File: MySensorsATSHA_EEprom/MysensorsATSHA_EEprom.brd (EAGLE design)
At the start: 22.1 x 12.1 mm, 3 parts, among them IC1 AT25DF512C-SSHN-B

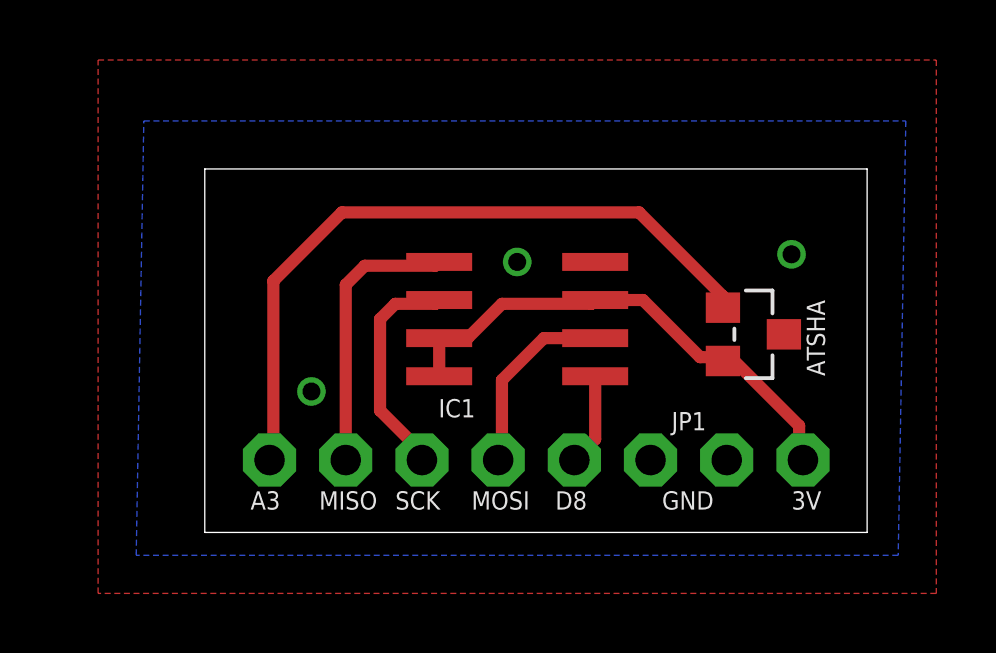
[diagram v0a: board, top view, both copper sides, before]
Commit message: routing minor changes
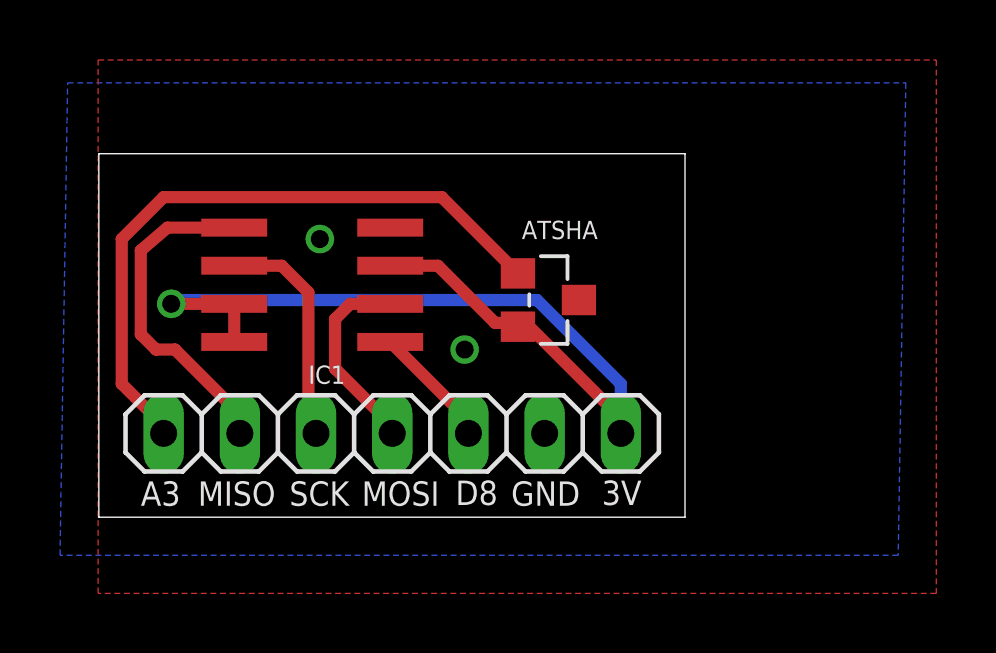
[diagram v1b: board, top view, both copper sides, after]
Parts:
- removed JP1: (no value), adafruit:1X08-CLEANBIG
- added JP2: (no value), pinhead:1X07
- moved ATSHA 6.93 mm to (15.0, 7.24)
- moved IC1 6.93 mm to (7.14, 7.75)
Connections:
- net A3: now also JP2.7; no longer JP1.8
- net D8: now also JP2.3; no longer JP1.4
- net GND: now also JP2.2; no longer JP1.2, JP1.3
- net MISO: now also JP2.6; no longer JP1.7
- net MOSI: now also JP2.4; no longer JP1.5
- net SCK: now also JP2.5; no longer JP1.6
- net VCC: now also JP2.1; no longer JP1.1
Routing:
- net VCC: track 16.7 -> 31.7 mm, vias 0 -> 1
- net MISO: track 9.27 -> 11.2 mm
- net A3: track 23.5 -> 21.9 mm
- net D8: track 3.08 -> 4.13 mm
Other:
- board size 22.1 x 12.1 mm -> 19.5 x 12.1 mm
